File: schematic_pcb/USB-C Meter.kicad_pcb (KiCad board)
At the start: 2 copper layers, 58.5 x 48 mm, 11 parts, among them J1 USB_C_Receptacle_PowerOnly_6P, J2 USB_C_Receptacle_PowerOnly_6P, U1 WEMOS_D1_mini, U2 INA226, U3 Display I2C

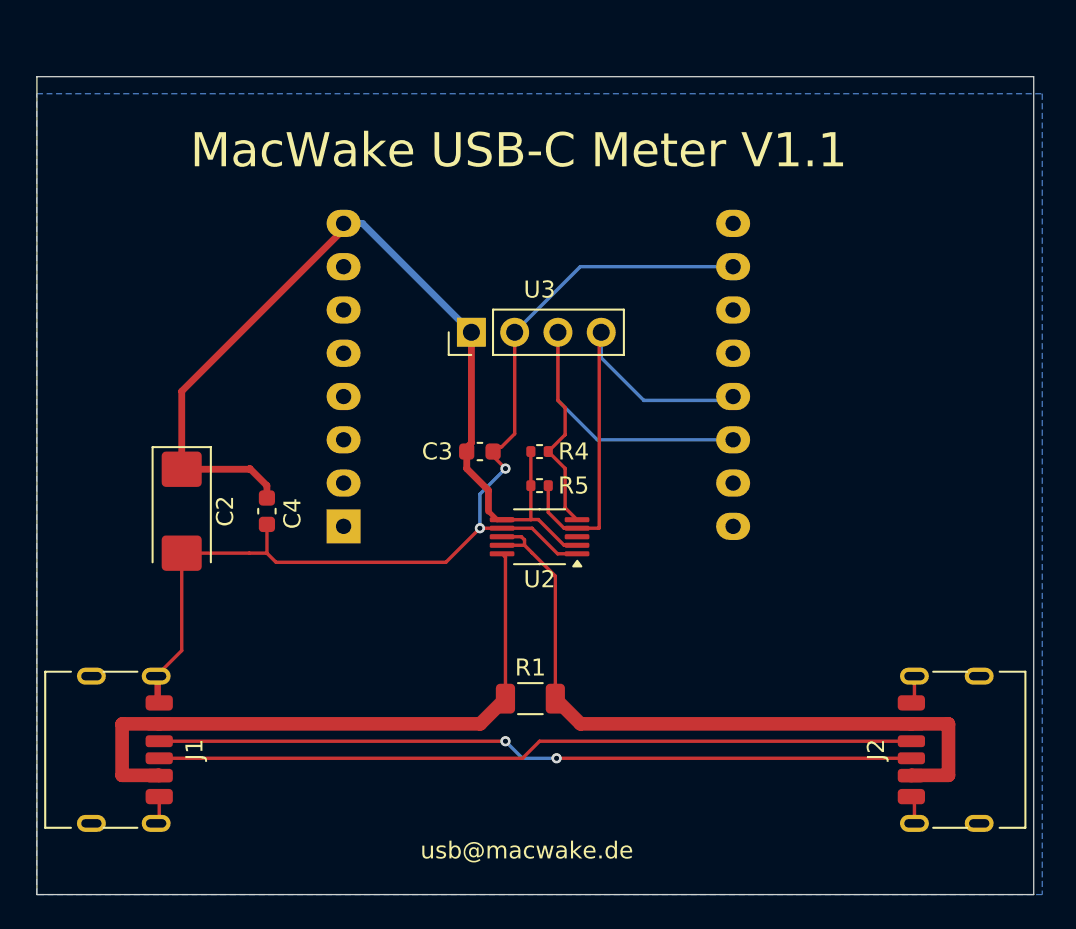
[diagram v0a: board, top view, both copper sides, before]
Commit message: feat: pcb/schematic v2.1.0
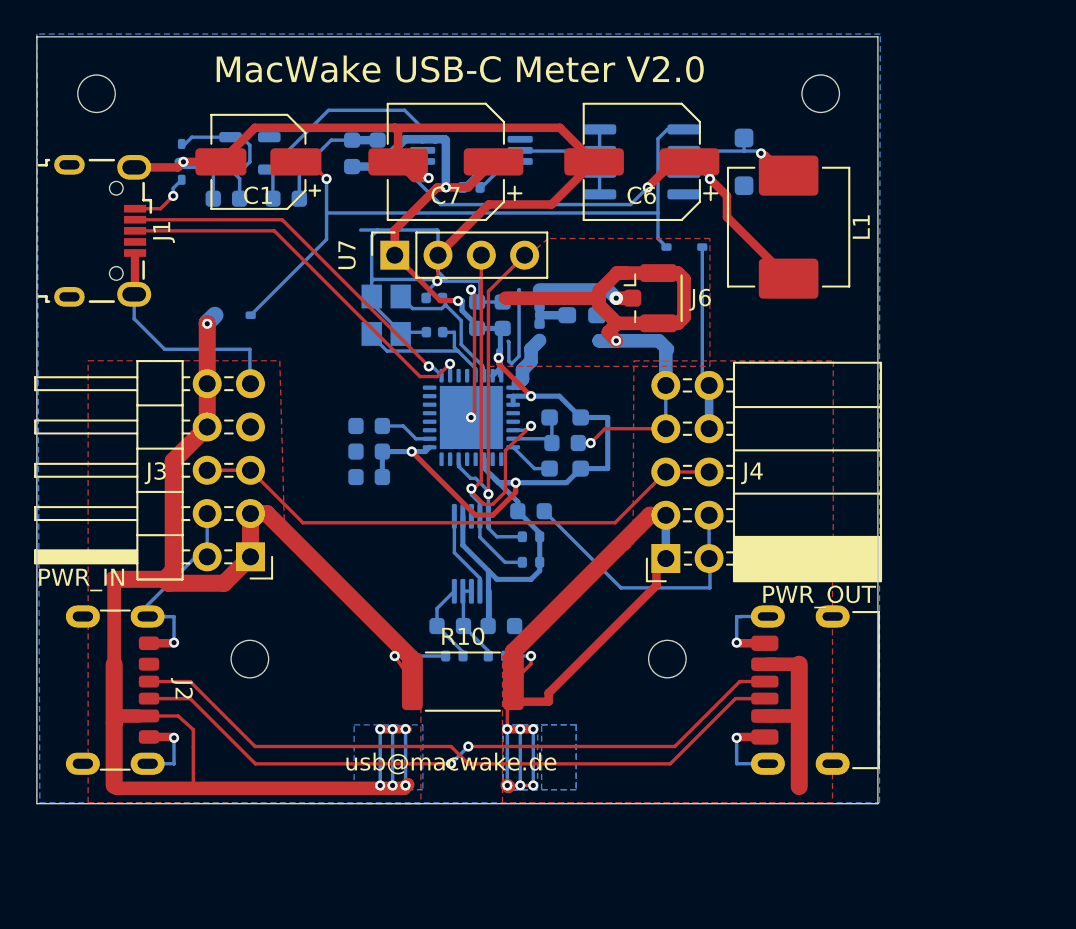
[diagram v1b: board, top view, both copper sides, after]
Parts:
- removed R5: 3k3, Resistor_SMD:R_0402_1005Metric
- added C1: 33µF/35V, Capacitor_SMD:CP_Elec_5x5.8, F.Cu at (71.5, 33.0)
- added C10: 0.1µ, Capacitor_SMD:C_0603_1608Metric, B.Cu at (87.5, 53.5)
- added C11: 1µ, Capacitor_SMD:C_0603_1608Metric, B.Cu at (78.0, 51.5)
- added C12: 0.1µ, Capacitor_SMD:C_0603_1608Metric, B.Cu at (78.0, 50.0)
- added C14: 1µ, Capacitor_SMD:C_0603_1608Metric, B.Cu at (84.3, 42.0)
- added C15: 10n, Capacitor_SMD:C_0603_1608Metric, B.Cu at (85.8, 42.0)
- added C16: 0.1µ, Capacitor_SMD:C_0603_1608Metric, B.Cu at (89.5, 49.5)
- added C17: 1pF, Capacitor_SMD:C_0402_1005Metric, B.Cu at (88.0, 43.0)
- added C18: 1pF, Capacitor_SMD:C_0402_1005Metric, B.Cu at (88.0, 41.0)
- added C20: 0.1µ, Capacitor_SMD:C_0603_1608Metric, B.Cu at (85.8, 60.2)
- added C21: 0.1µ, Capacitor_SMD:C_0603_1608Metric, B.Cu at (82.8, 60.2)
- added C3: 10µF, Capacitor_SMD:C_0603_1608Metric, B.Cu at (73.1, 35.2)
- added C5: 10pF, Capacitor_SMD:C_0402_1005Metric, B.Cu at (81.8, 41.0)
- added C6: 220µF, Capacitor_SMD:CP_Elec_6.3x5.9, F.Cu at (94.0, 33.0)
- added C7: 220µF, Capacitor_SMD:CP_Elec_6.3x5.9, F.Cu at (82.5, 33.0)
- added C8: 0.1µ, Capacitor_SMD:C_0603_1608Metric, B.Cu at (77.0, 32.5)
- added C9: 10µF, Capacitor_SMD:C_0603_1608Metric, B.Cu at (78.5, 32.5)
- added D1: 1N5819WS, Diode_SMD:D_SOD-323, B.Cu at (67.0, 33.0)
- added D2: PMEG2005EH, Diode_SMD:D_SOD-123F, B.Cu at (100.0, 33.0)
- added D3: 1N5819WS, Diode_SMD:D_SOD-323, B.Cu at (70.0, 42.0)
- added D4: 1N5819WS, Diode_SMD:D_SOD-323, B.Cu at (96.5, 38.0)
- added J1: USB_B_Micro, Connector_USB:USB_Micro-B_Wuerth_629105150521, F.Cu at (62.4, 37.0)
- added J3: Generic IN, Connector_PinHeader_2.54mm:PinHeader_2x05_P2.54mm_Horizontal, F.Cu at (71.0, 56.2)
- added J4: Generic OUT, Connector_PinSocket_2.54mm:PinSocket_2x05_P2.54mm_Horizontal, F.Cu at (95.4, 56.3)
- added J6: Conn_Coaxial, Connector_Coaxial:U.FL_Hirose_U.FL-R-SMT-1_Vertical, F.Cu at (94.5, 41.0)
- added L1: 47µH, Inductor_SMD:L_Changjiang_FXL0630, F.Cu at (102.6, 36.8)
- added L2: 2.7nH, Inductor_SMD:L_0603_1608Metric_Pad1.05x0.95mm_HandSolder, B.Cu at (90.5, 42.0)
- added R10: 0.01R 3W, Resistor_SMD:R_2512_6332Metric, F.Cu at (83.5, 63.5)
- added R11: 10R, Resistor_SMD:R_0402_1005Metric, B.Cu at (85.5, 62.0)
- added R12: 12k, Resistor_SMD:R_0603_1608Metric_Pad0.98x0.95mm_HandSolder, B.Cu at (89.5, 51.0)
- added R2: 3k3, Resistor_SMD:R_0402_1005Metric, B.Cu at (87.5, 55.0)
- added R3: 400R, Resistor_SMD:R_0402_1005Metric, B.Cu at (84.0, 34.5)
- added R9: 10R, Resistor_SMD:R_0402_1005Metric, B.Cu at (83.0, 62.0)
- added REF**: MountingHole_2.2mm_M2_DIN965, MountingHole:MountingHole_2.2mm_M2_DIN965, F.Cu at (95.5, 62.2)
- added REF**: MountingHole_2.2mm_M2_DIN965, MountingHole:MountingHole_2.2mm_M2_DIN965, F.Cu at (62.0, 29.0)
- added REF**: MountingHole_2.2mm_M2_DIN965, MountingHole:MountingHole_2.2mm_M2_DIN965, F.Cu at (71.0, 62.2)
- added REF**: MountingHole_2.2mm_M2_DIN965, MountingHole:MountingHole_2.2mm_M2_DIN965, F.Cu at (104.5, 29.0)
- added U2: ME6211C33M5, Package_TO_SOT_SMD:SOT-23-5, B.Cu at (71.0, 32.5)
- added U3: TPS2115, Package_SO:TSSOP-8_4.4x3mm_P0.65mm, B.Cu at (84.0, 32.0)
- added U4: ESP32-C3FH4, Package_DFN_QFN:QFN-32-1EP_5x5mm_P0.5mm_EP3.7x3.7mm, B.Cu at (84.0, 48.0)
- added Y1: 40MHz, Crystal:Crystal_SMD_3225-4Pin_3.2x2.5mm, B.Cu at (79.0, 42.0)
- C13: renamed from C3; moved to B.Cu
- C2: value 20µ -> 10µF; footprint Capacitor_Tantalum_SMD:CP_EIA-6032-20_AVX-F -> Capacitor_SMD:C_0603_1608Metric; moved to B.Cu
- C4: value 0.1µ -> 10pF; footprint Capacitor_SMD:C_0603_1608Metric -> Capacitor_SMD:C_0402_1005Metric; moved to B.Cu
- J2: renamed from J1; value USB_C_Receptacle_PowerOnly_6P -> USB-C Receptacle 6P; footprint Connector_USB:USB_C_Receptacle_HRO_TYPE-C-31-M-17 -> Connector_USB:USB_C_Receptacle_GCT_USB4125-xx-x_6P_TopMnt_Horizontal
- J5: renamed from J2; value USB_C_Receptacle_PowerOnly_6P -> USB-C Receptacle 6P
- R1: value 0.01R 3W -> 3k3; footprint Resistor_SMD:R_1206_3216Metric -> Resistor_SMD:R_0402_1005Metric; moved to B.Cu
- R4: value 3k3 -> 12k; footprint Resistor_SMD:R_0402_1005Metric -> Resistor_SMD:R_0603_1608Metric_Pad0.98x0.95mm_HandSolder; moved to B.Cu
- U1: value WEMOS_D1_mini -> XL1509-3.3; footprint RF_Module:WEMOS_D1_mini_light -> Package_SO:SOIC-8_3.9x4.9mm_P1.27mm
- U6: renamed from U2; value INA226 -> INA228; moved to B.Cu
- U7: renamed from U3; footprint Connector_PinHeader_2.54mm:PinHeader_1x04_P2.54mm_Vertical -> Connector_PinSocket_2.54mm:PinSocket_1x04_P2.54mm_Vertical
- moved U1 27.6 mm to (94.0, 33.0), turned to 180 degrees
- moved C2 18.5 mm to (69.6, 35.2), turned to 180 degrees
- moved C4 14.4 mm to (81.8, 43.0), turned to 180 degrees
- moved J5 9.28 mm to (104.4, 64.0)
- moved R1 8.00 mm to (87.5, 56.5)
- moved C13 6.67 mm to (78.0, 48.5)
- moved U7 6.38 mm to (79.5, 38.5)
- moved U6 4.12 mm to (84.0, 56.0), turned to -90 degrees
- moved J2 3.54 mm to (62.0, 64.0)
- moved R4 2.50 mm to (89.5, 48.0), turned to 0 degrees
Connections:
- net Net-(J1-CC1) renamed /CC1
- net Net-(J1-CC2) renamed /CC2
- C13 pad 1: Net-(U1-3V3) -> GND
- C13 pad 2: Net-(J1-SHIELD) -> Net-(U4-VDD_SPI)
- C2 pad 1: Net-(U1-3V3) -> /VBUS_DATA_R
- C2 pad 2: Net-(J1-SHIELD) -> GND
- C4 pad 1: Net-(J1-SHIELD) -> Net-(U4-XTAL_N)
- C4 pad 2: Net-(U1-3V3) -> GND
- J2 pad A12: Net-(J1-SHIELD) -> GND
- J2 pad A9: Net-(U2-Vin+) -> /VBUS_PD_1_IN
- J2 pad B12: Net-(J1-SHIELD) -> GND
- J2 pad B9: Net-(U2-Vin+) -> /VBUS_PD_1_IN
- J2 pad S1: Net-(J1-SHIELD) -> GND
- J5 pad A12: Net-(J1-SHIELD) -> GND
- J5 pad A9: Net-(U2-Vbus) -> /VBUS_PD_2_IN
- J5 pad B12: Net-(J1-SHIELD) -> GND
- J5 pad B9: Net-(U2-Vbus) -> /VBUS_PD_2_IN
- J5 pad S1: Net-(J1-SHIELD) -> GND
- R1 pad 1: Net-(U2-Vin+) -> SDA
- R1 pad 2: Net-(U2-Vbus) -> 3V3
- R4 pad 1: Net-(U1-SCL/D1) -> Net-(U4-CHIP_EN)
- R4 pad 2: Net-(U1-3V3) -> 3V3
- U1 pad 1: unconnected-(U1-~{RST}-Pad1) -> /VBUS_PD_R
- U1 pad 2: unconnected-(U1-A0-Pad2) -> Net-(D2-K)
- U1 pad 3: unconnected-(U1-D0-Pad3) -> /VBUS_PD_3V3
- U1 pad 4: unconnected-(U1-SCK/D5-Pad4) -> GND
- U1 pad 5: unconnected-(U1-MISO/D6-Pad5) -> GND
- U1 pad 6: unconnected-(U1-MOSI/D7-Pad6) -> GND
- U1 pad 7: unconnected-(U1-CS/D8-Pad7) -> GND
- U1 pad 8: Net-(U1-3V3) -> GND
- U6 pad 1: Net-(J1-SHIELD) -> GND
- U6 pad 10: Net-(U2-Vin+) -> /SHNT+
- U6 pad 2: Net-(U1-3V3) -> 3V3
- U6 pad 4: Net-(U1-SDA/D2) -> SDA
- U6 pad 5: Net-(U1-SCL/D1) -> SCL
- U6 pad 6: Net-(U1-3V3) -> 3V3
- U6 pad 7: Net-(J1-SHIELD) -> GND
- U6 pad 8: Net-(U2-Vbus) -> /SHNT-
- U6 pad 9: Net-(U2-Vbus) -> /SHNT-
- U7 pad 1: Net-(U1-3V3) -> 3V3
- U7 pad 2: Net-(J1-SHIELD) -> GND
- U7 pad 3: Net-(U1-SCL/D1) -> SDA
- U7 pad 4: Net-(U1-SDA/D2) -> SCL
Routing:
- net GND: track 0.00 -> 221.5 mm, vias 0 -> 11
- net /VBUS_PD_1_IN: track 0.00 -> 111.7 mm, vias 0 -> 8
- net 3V3: track 0.00 -> 84.6 mm, vias 0 -> 6
- net Net-(J1-SHIELD): track 70.5 -> 0.00 mm, vias 2 -> 0
- net /VBUS_PD_2_IN: track 0.00 -> 70.4 mm, vias 0 -> 7
- net Net-(U1-3V3): track 57.0 -> 0.00 mm
- net Net-(U2-Vbus): track 41.1 -> 0.00 mm
- net /VBUS_PD_R: track 0.00 -> 39.0 mm, vias 0 -> 1
- net Net-(U2-Vin+): track 36.9 -> 0.00 mm
- net /CHGR_ID_GENERIC: track 0.00 -> 32.0 mm
- net /VBUS_PD_3V3: track 0.00 -> 29.2 mm, vias 0 -> 2
- net SDA: track 0.00 -> 28.6 mm, vias 0 -> 2
- net Net-(U1-SCL/D1): track 27.5 -> 0.00 mm
- net Net-(U1-SDA/D2): track 27.1 -> 0.00 mm
- net Net-(J1-D+): track 0.00 -> 23.0 mm, vias 0 -> 1
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- added copper zone on B.Cu, net /VBUS_PD_1_IN
- added copper zone on F.Cu, net /VBUS_PD_1_IN
- added copper zone on B.Cu, net /VBUS_PD_2_IN
- added copper zone on F.Cu, net /VBUS_PD_2_IN
- added copper zone on B.Cu, net GND
- added copper zone on F.Cu, net GND
- removed copper zone on B.Cu, net Net-(J1-SHIELD)
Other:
- board size 58.5 x 48 mm -> 49.4 x 45 mm
- board text added: "MacWake USB-C Meter V2.0"
- board text added: "PWR_IN"
- board text added: "PWR_OUT"
- board text removed: "MacWake USB-C Meter V1.1"
